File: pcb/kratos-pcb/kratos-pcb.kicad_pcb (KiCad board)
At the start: 2 copper layers, 100 x 100 mm, 29 parts, among them IC2 SN74HC595N, J1 Barrel_Jack_Switch_Pin3Ring, Q2 2N2222A, Q3 2N2222A, SW1 SW_Push, U1 ESP32-DEVKIT-V1, U2 ULN2803A, U3 ULN2803A

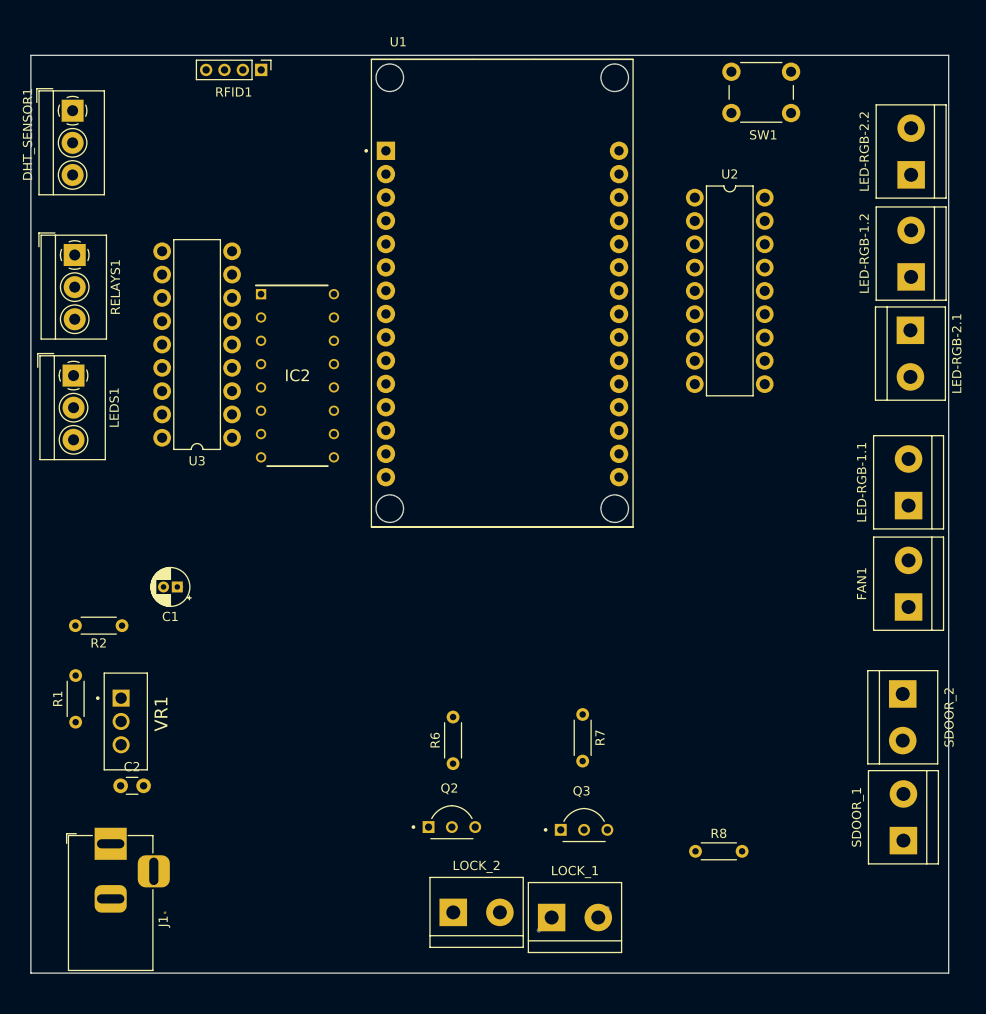
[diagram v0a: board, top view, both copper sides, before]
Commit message: ### added
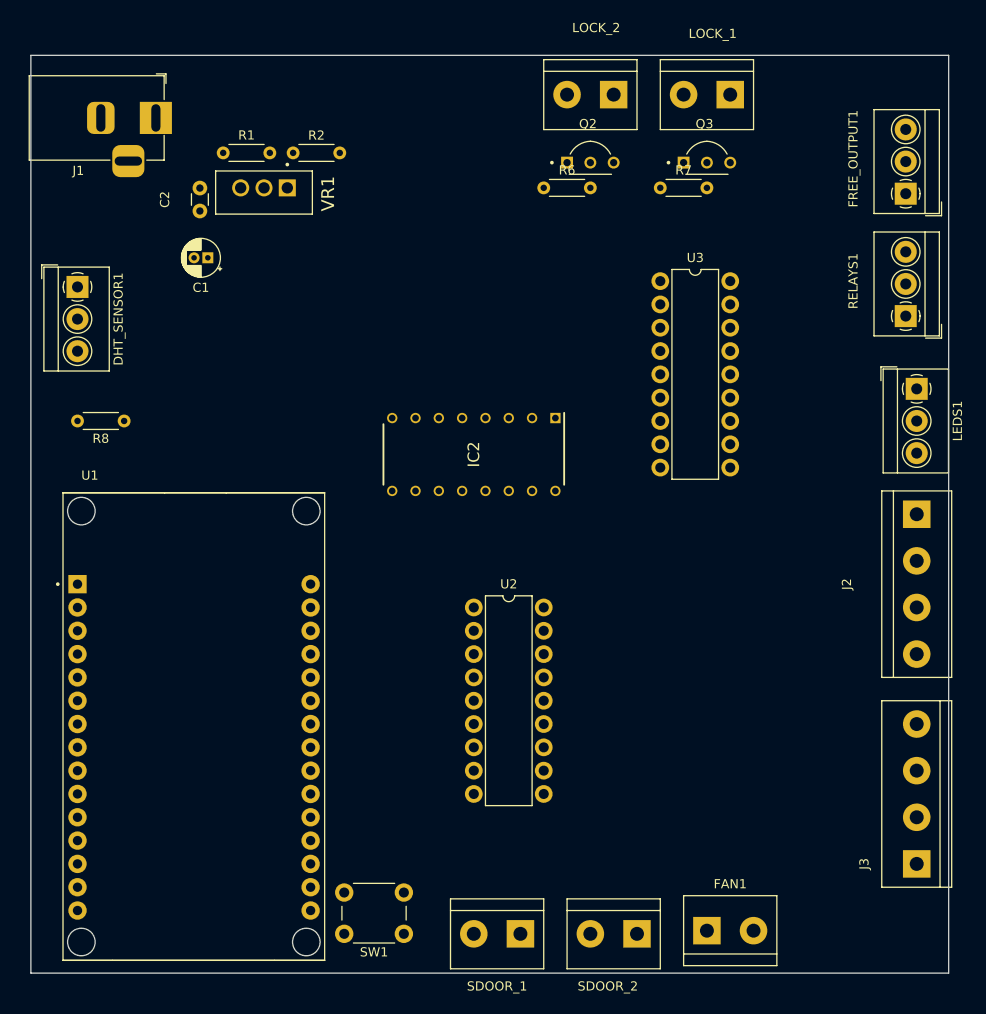
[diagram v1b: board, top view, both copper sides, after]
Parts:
- removed LED-RGB-1.1, LED-RGB-1.2, LED-RGB-2.1, LED-RGB-2.2: Screw_Terminal_01x02, TerminalBlock:TerminalBlock_bornier-2_P5.08mm
- removed RFID1: Conn_01x04_Pin, Connector_PinHeader_2.00mm:PinHeader_1x04_P2.00mm_Vertical
- added FREE_OUTPUT1: Screw_Terminal_01x03, TerminalBlock_4Ucon:TerminalBlock_4Ucon_1x03_P3.50mm_Horizontal, F.Cu at (189.3, 59.1)
- added J2: Screw_Terminal_01x04, TerminalBlock:TerminalBlock_bornier-4_P5.08mm, F.Cu at (190.5, 94.0)
- added J3: Screw_Terminal_01x04, TerminalBlock:TerminalBlock_bornier-4_P5.08mm, F.Cu at (190.5, 132.1)
- moved SW1 100.5 mm to (134.6, 139.7), turned to 180 degrees
- moved LEDS1 91.9 mm to (190.5, 80.3)
- moved LOCK_1 91.7 mm to (170.2, 48.3), turned to 180 degrees
- moved LOCK_2 90.8 mm to (157.5, 48.3), turned to 180 degrees
- moved RELAYS1 90.8 mm to (189.3, 72.4), turned to 90 degrees
- moved J1 79.2 mm to (107.6, 50.8), turned to 0 degrees
- moved R8 77.9 mm to (104.1, 83.8), turned to 180 degrees
- moved Q2 74.0 mm to (154.9, 53.3)
- moved Q3 73.9 mm to (167.6, 53.3)
- moved C2 65.7 mm to (112.4, 58.4), turned to -90 degrees
- moved R1 64.1 mm to (114.9, 54.6), turned to 0 degrees
- moved R6 63.5 mm to (149.9, 58.4), turned to 0 degrees
- moved VR1 60.2 mm to (119.4, 58.4), turned to 180 degrees
- moved R7 58.0 mm to (162.6, 58.4), turned to 0 degrees
- moved U1 58.0 mm to (111.8, 117.1)
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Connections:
- LOCK_1 pad 1: +12V -> Net-(LOCK_1-Pin_1)
- LOCK_1 pad 2: Net-(LOCK_1-Pin_2) -> +12V
- LOCK_2 pad 1: +12V -> Net-(LOCK_2-Pin_1)
- LOCK_2 pad 2: Net-(LOCK_2-Pin_2) -> +12V
- Q2 pad 3: Net-(LOCK_2-Pin_2) -> Net-(LOCK_2-Pin_1)
- Q3 pad 3: Net-(LOCK_1-Pin_2) -> Net-(LOCK_1-Pin_1)
- U2 pad 1: GREEN-LED-2 -> RED-LED
- U2 pad 2: RED-LED-2 -> GREEN-LED
- U2 pad 3: BLUE-LED-2 -> BLUE-LED
- U2 pad 4: RED-LED -> RED-LED-2
- U2 pad 5: GREEN-LED -> GREEN-LED-2
- U2 pad 6: BLUE-LED -> BLUE-LED-2
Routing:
- net +12V: track 2.20 -> 0.00 mm
- net Net-(LOCK_1-Pin_2): track 1.40 -> 0.00 mm
- net +5V: track 0.51 -> 0.00 mm
